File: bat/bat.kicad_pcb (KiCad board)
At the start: 2 copper layers, 87.2 x 49.4 mm, 19 parts, among them Q1 2N3904, Q2 2N3904, Q3 S8550, SW1 SW_SPDT

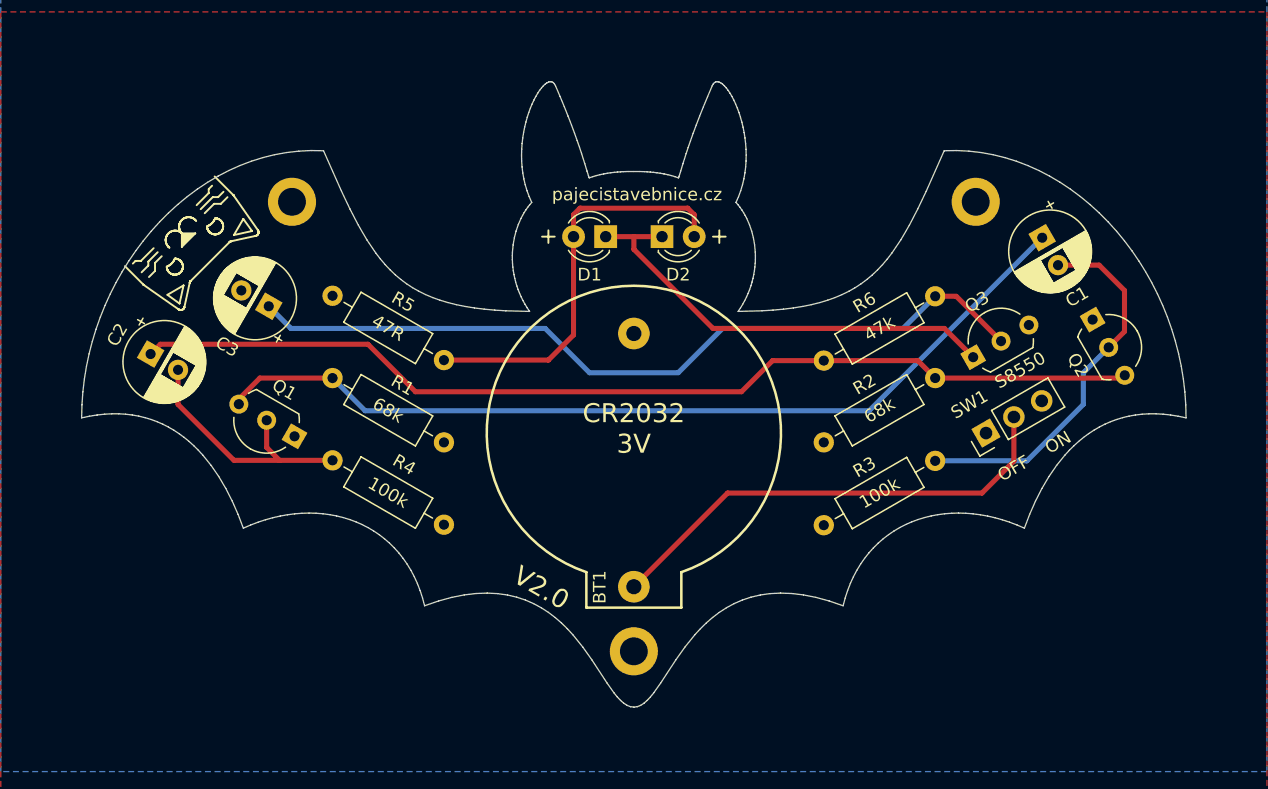
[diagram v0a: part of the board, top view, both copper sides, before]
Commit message: Bat V2.1, mddm-badge tooling added
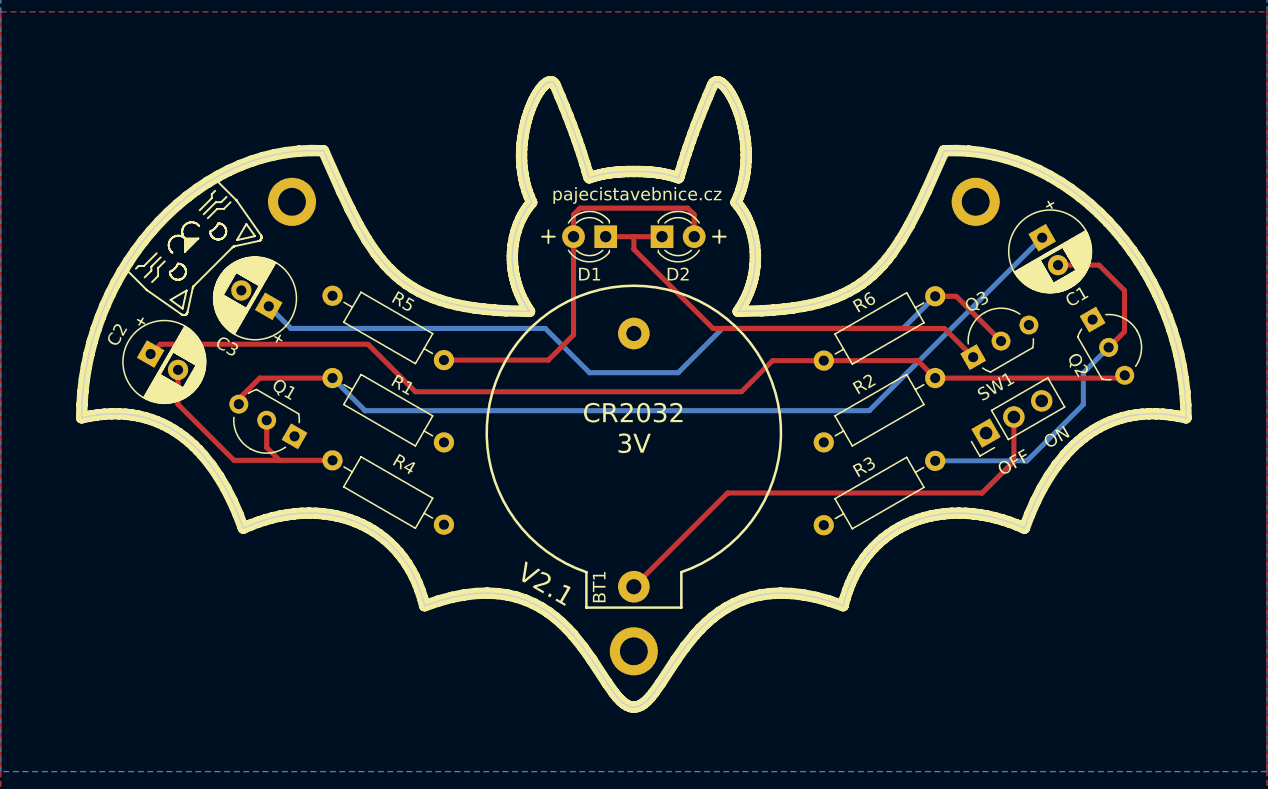
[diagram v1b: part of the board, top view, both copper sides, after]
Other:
- board text added: "V2.1"
- board text removed: "100k"
- board text removed: "47R"
- board text removed: "47k"
- board text removed: "68k"
- board text removed: "S8550"
- board text removed: "V2.0"
